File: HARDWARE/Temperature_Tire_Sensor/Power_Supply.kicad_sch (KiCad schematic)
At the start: 8 parts

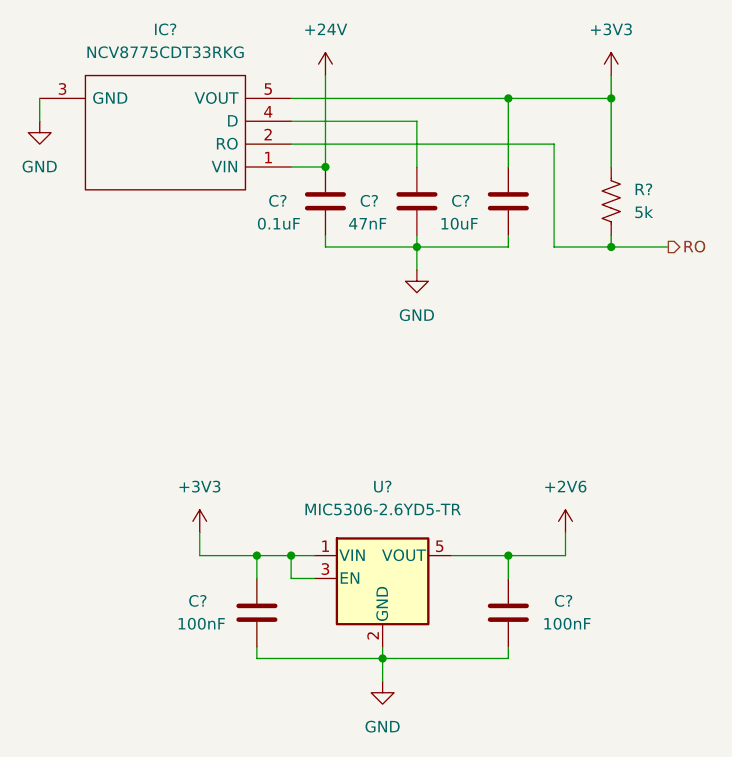
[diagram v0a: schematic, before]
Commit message: A completed schematic
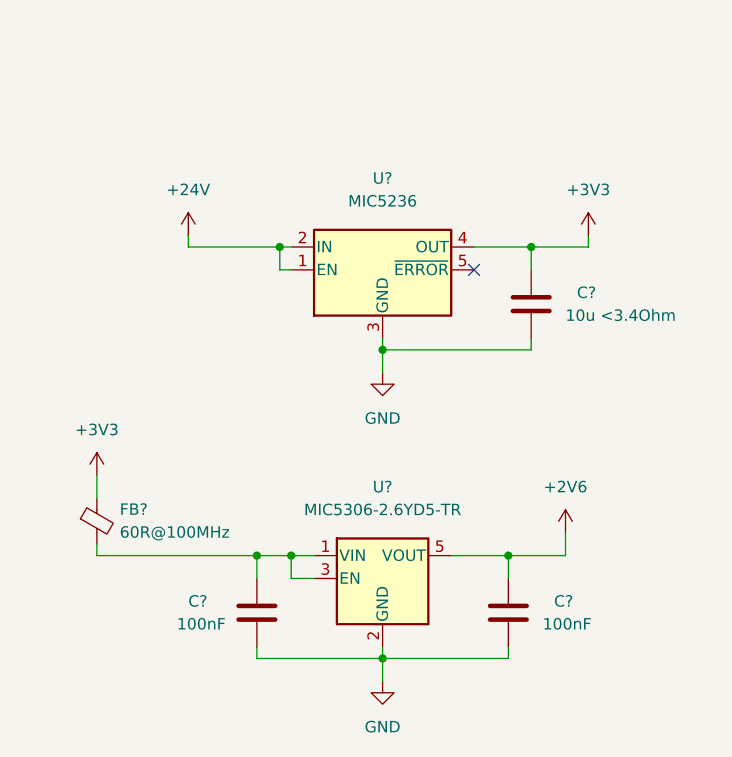
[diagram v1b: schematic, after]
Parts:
- removed C?: 0.1uF, symbol Device:C
- removed C?: 47nF, symbol Device:C
- removed C?: 10uF, symbol Device:C
- removed IC?: NCV8775CDT33RKG, NCV8775CDT33RKG, symbol NCV8775CDT33RKG:NCV8775CDT33RKG
- removed R?: 5k, symbol Device:R_US
- added C?: 10u <3.4Ohm, symbol Device:C
- added FB?: 60R@100MHz, symbol Device:FerriteBead_Small
- added U?: MIC5236, symbol Regulator_Linear:LP38512TJ-1.8
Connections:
- net +24V: now also U?.1 (EN), U?.2 (IN)
- net +3V3: now also C?.1, FB?.1, U?.4 (OUT); no longer C?.1, U?.1 (VIN), U?.3 (EN)
- net GND: now also C?.2, U?.3 (GND), U?.6 (GND)
- new net: C?.1, FB?.2, U?.1 (VIN), U?.3 (EN)
- no-connect marks 0 -> 1
